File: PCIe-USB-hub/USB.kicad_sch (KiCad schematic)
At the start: 8 parts, among them J2 USB3_A_Stacked, J3 USB3_A_Stacked, J4 USB3_A_Stacked, J5 USB3_A_Stacked, J6 USB3_A_Stacked, J7 USB3_A_Stacked, J8 USB3_A_Stacked, J9 USB3_A_Stacked

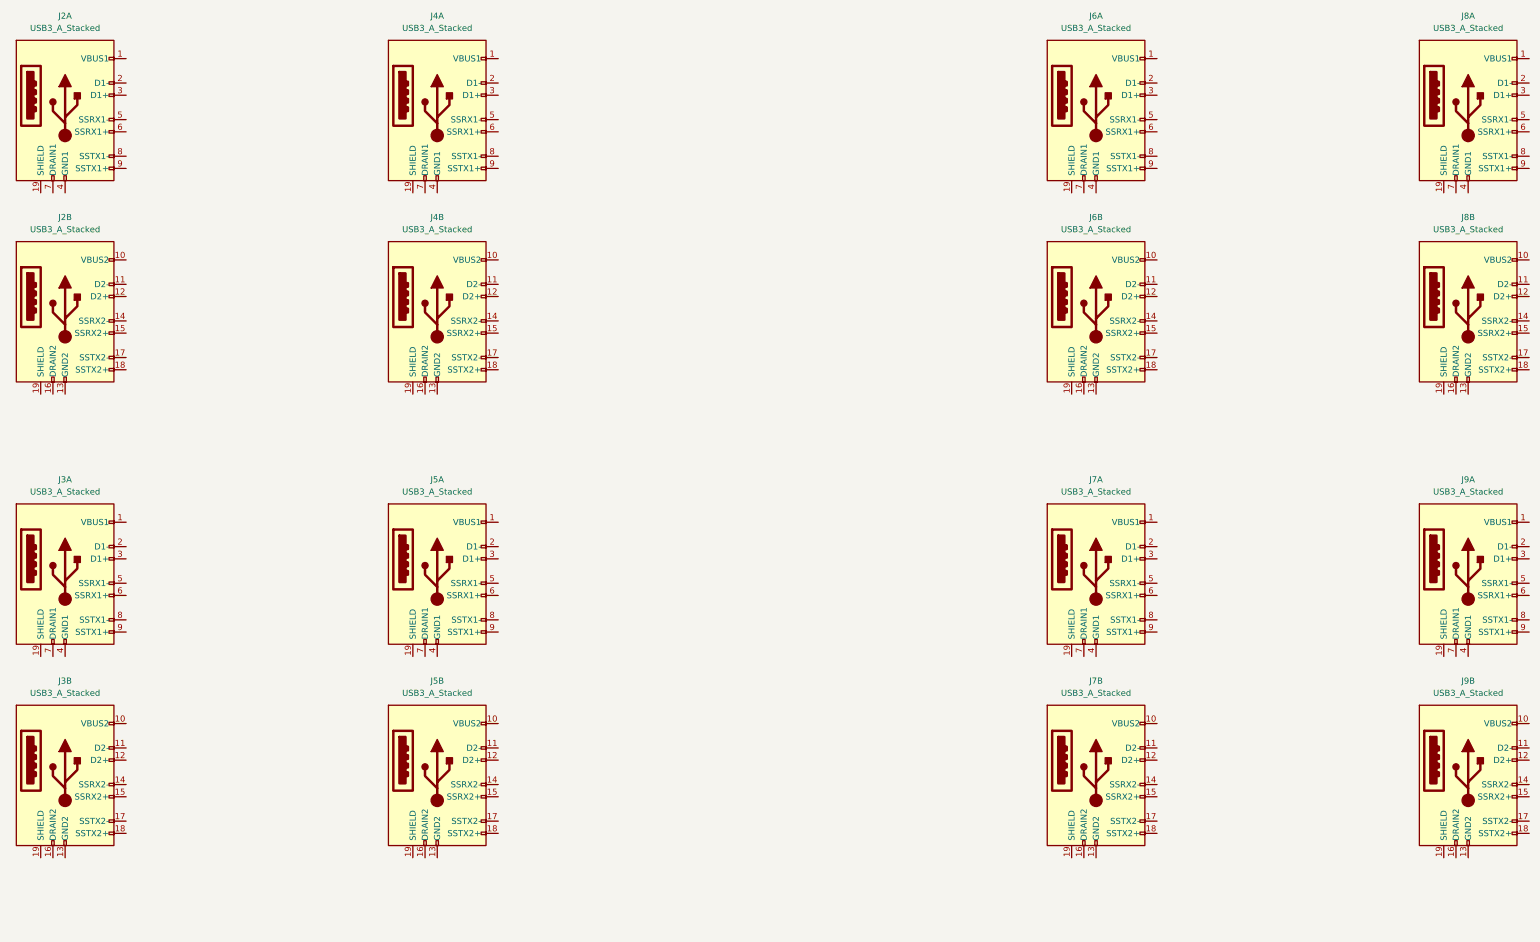
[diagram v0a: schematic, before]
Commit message: Частично добавил компоненты
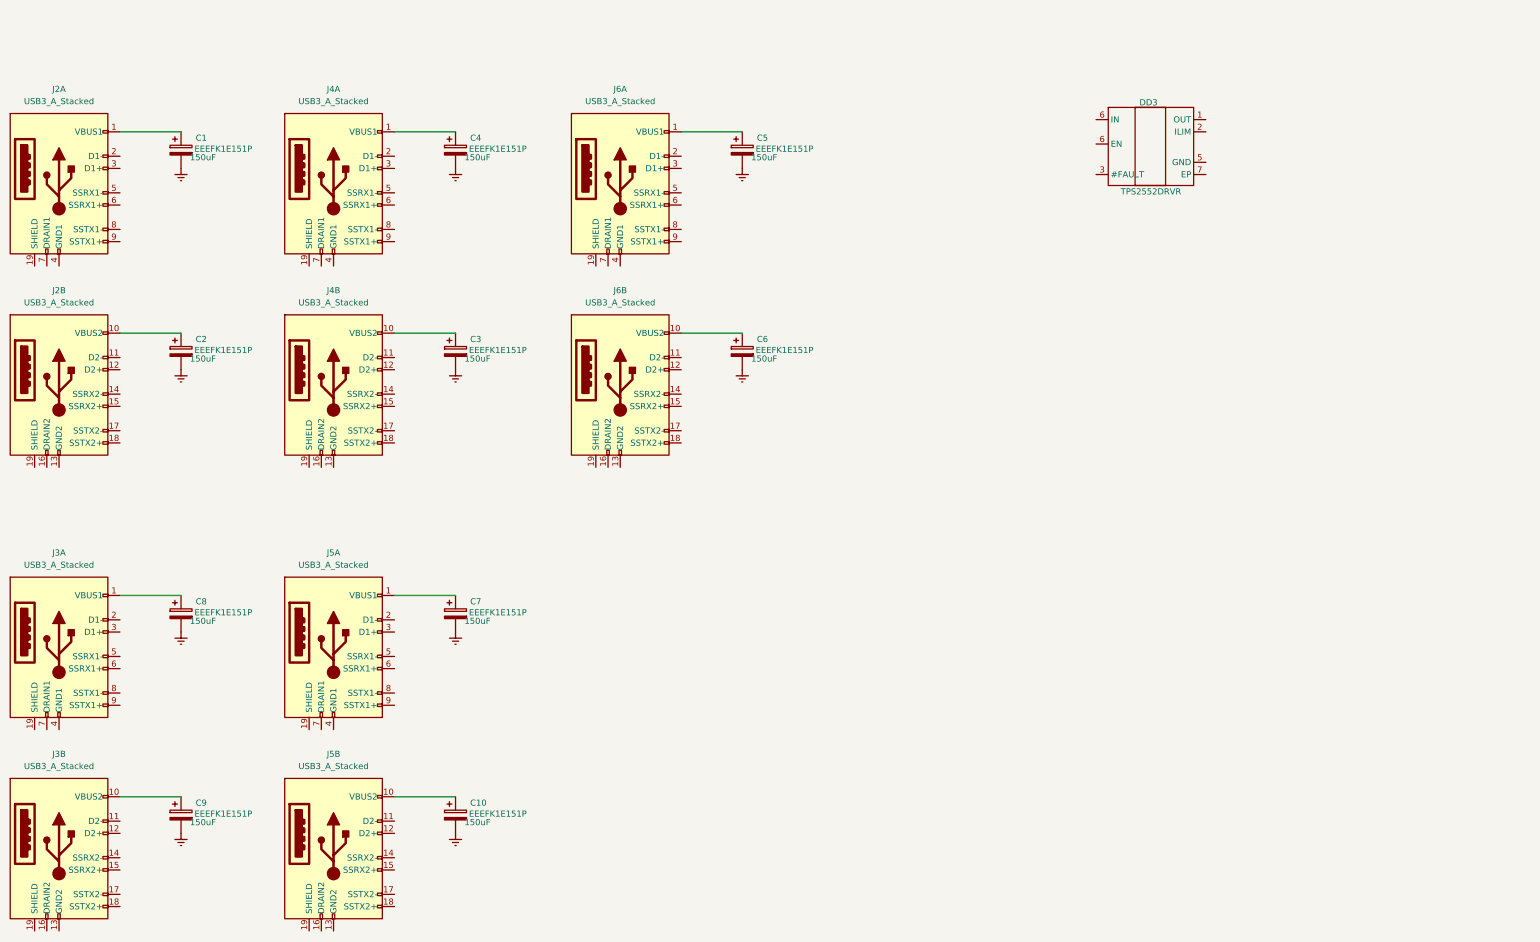
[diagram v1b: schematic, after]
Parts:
- removed J7, J8, J9: USB3_A_Stacked, Connector_USB:USB3_A_Molex_48406-0001_Horizontal_Stacked, symbol Connector:USB3_A_Stacked
- added C1, C10, C2, C3, C4, C5, C6, C7, C8, C9: EEEFK1E151P, Capacitor_SMD:C_Elec_8x10.2, symbol Device:C_Polarized
- added DD3: TPS2552DRVR, Package_SON:WSON-6-1EP_2x2mm_P0.65mm_EP1x1.6mm, symbol TPS2552DRVR:TPS2552DRVR
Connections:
- net at J4.10 (VBUS2): now also C3.1
- net at J3.10 (VBUS2): now also C9.1
- net at J6.10 (VBUS2): now also C6.1
- net at J5.1 (VBUS1): now also C7.1
- net at J5.10 (VBUS2): now also C10.1
- net at J6.1 (VBUS1): now also C5.1
- net at J2.10 (VBUS2): now also C2.1
- net at J3.1 (VBUS1): now also C8.1
- net at J4.1 (VBUS1): now also C4.1
- net at J2.1 (VBUS1): now also C1.1
- new net Earth: C1.2, C10.2, C2.2, C3.2, C4.2, C5.2, C6.2, C7.2, C8.2, C9.2
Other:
- moved on the sheet: J2A, J2B, J3A, J3B, J4A, J4B, J5A, J5B, J6A, J6B
